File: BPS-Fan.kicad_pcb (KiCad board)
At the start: 2 copper layers, 34.3 x 41.2 mm, 33 parts, among them J1 LDRBRDConn, J2 FAN7, J3 FAN7, J4 FAN7, J5 FAN7, Q3 IRLML0030, Q6 IRLML0030, Q7 IRLML0030, Q8 IRLML0030

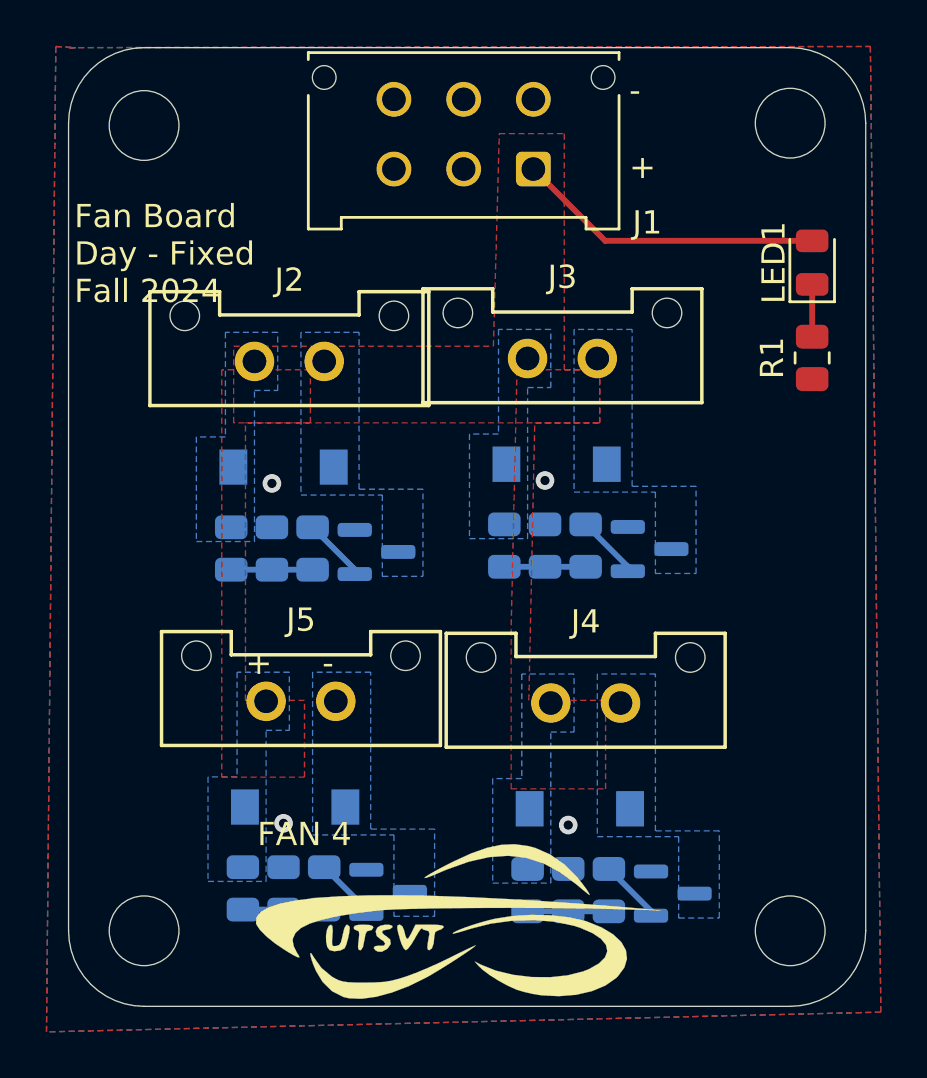
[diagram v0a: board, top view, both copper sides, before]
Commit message: done
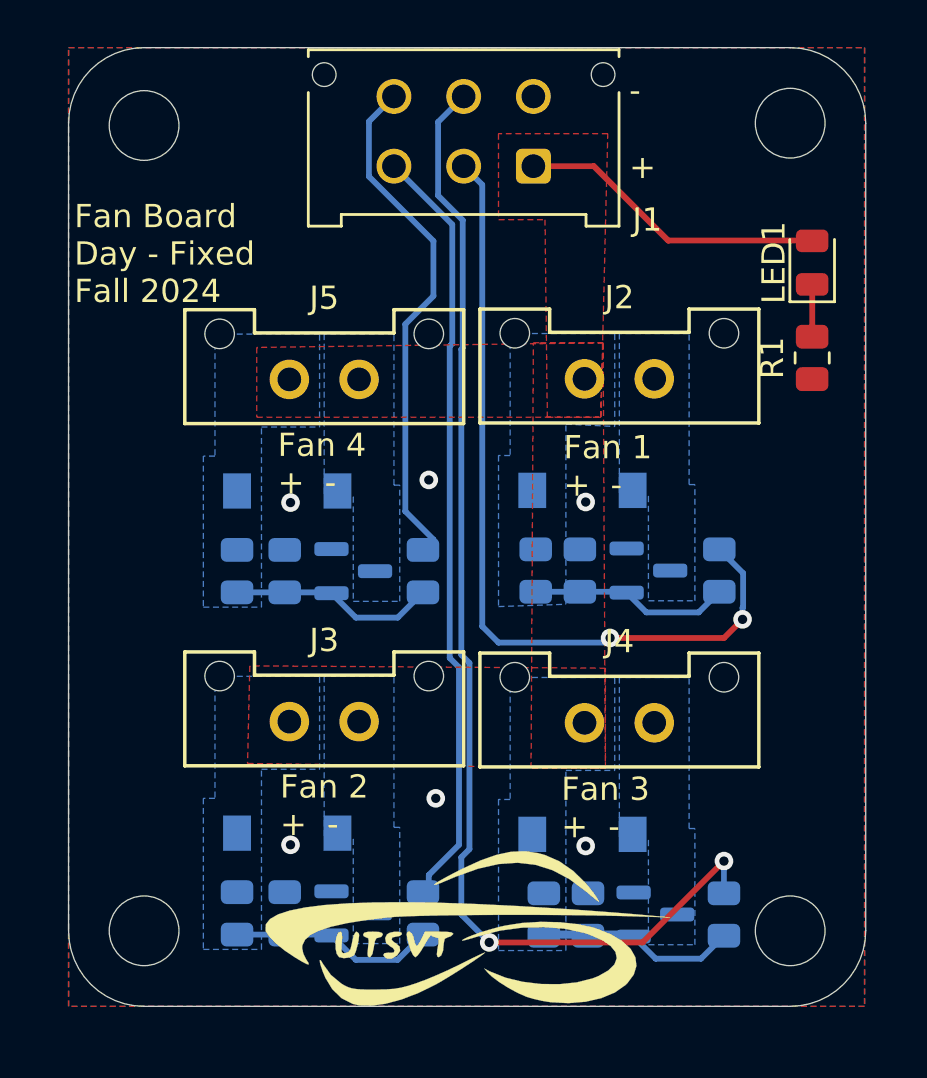
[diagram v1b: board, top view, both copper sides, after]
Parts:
- moved Q6 20.2 mm to (133.1, 95.1)
- moved D2 19.7 mm to (130.3, 91.6)
- moved R5 19.6 mm to (128.1, 95.1)
- moved R6 19.4 mm to (130.2, 95.1)
- moved J3 18.7 mm to (130.4, 86.8)
- moved R4 17.5 mm to (148.9, 80.3), turned to -90 degrees
- moved R8 17.3 mm to (136.1, 95.1), turned to -90 degrees
- moved R13 14.3 mm to (136.1, 80.3), turned to -90 degrees
- moved J2 14.2 mm to (143.1, 72.1)
- moved J5 13.9 mm to (130.4, 72.1)
- moved Q8 13.9 mm to (133.1, 80.3)
- moved R10 13.7 mm to (128.1, 80.3)
- moved R11 13.7 mm to (130.2, 80.3)
- moved D5 13.6 mm to (130.3, 76.9)
- moved R3 13.3 mm to (142.9, 80.3)
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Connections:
- R10 pad 2: /FAN4_BPS -> Net-(Q8-G)
- R11 pad 2: /FAN4_BPS -> Net-(Q8-G)
- R2 pad 2: /FAN1_BPS -> Net-(Q3-G)
- R3 pad 2: /FAN1_BPS -> Net-(Q3-G)
- R5 pad 2: /FAN2_BPS -> Net-(Q6-G)
- R6 pad 2: /FAN2_BPS -> Net-(Q6-G)
- R7 pad 2: /FAN3_BPS -> Net-(Q7-G)
- R9 pad 2: /FAN3_BPS -> Net-(Q7-G)
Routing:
- net /FAN3_BPS: track 3.50 -> 51.0 mm, vias 0 -> 2
- net /FAN1_BPS: track 3.50 -> 35.5 mm, vias 0 -> 2
- net /FAN2_BPS: track 3.50 -> 33.0 mm
- net /FAN4_BPS: track 3.50 -> 22.3 mm
- net Net-(Q7-G): track 2.76 -> 12.6 mm
- net Net-(Q6-G): track 2.76 -> 8.90 mm
- net Net-(Q8-G): track 2.76 -> 8.90 mm
- net Net-(Q3-G): track 2.76 -> 8.64 mm
- net GNDPWR: vias 4 -> 6
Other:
- board text added: "Fan 1 + -"
- board text added: "Fan 2 + -"
- board text added: "Fan 3 + -"
- board text added: "Fan 4 + -"
- board text removed: "FAN 4"
